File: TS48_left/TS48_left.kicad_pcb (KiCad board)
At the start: 2 copper layers, 124 x 77.9 mm, 123 parts, among them Q1 Q_NPN_BCE, SW1 SW_PUSH, U1 ATmega32U4, U2 PRTR5V0U2X, Y1 

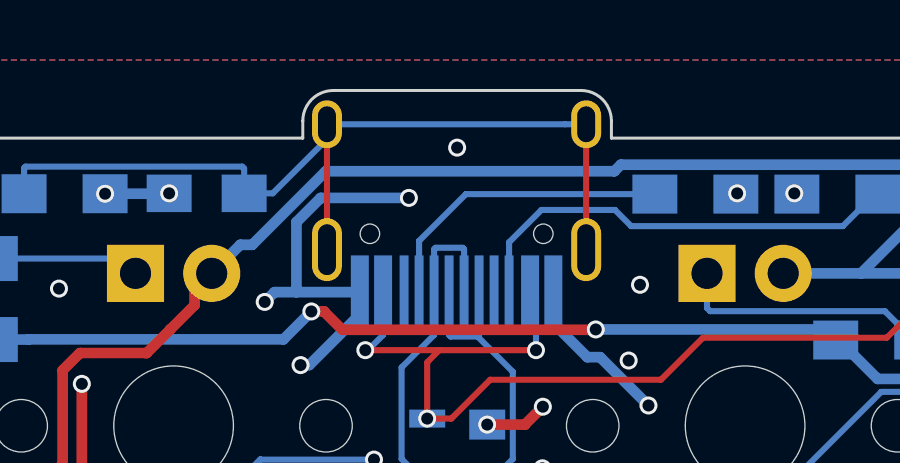
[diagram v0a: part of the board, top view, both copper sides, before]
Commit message: Gerbers
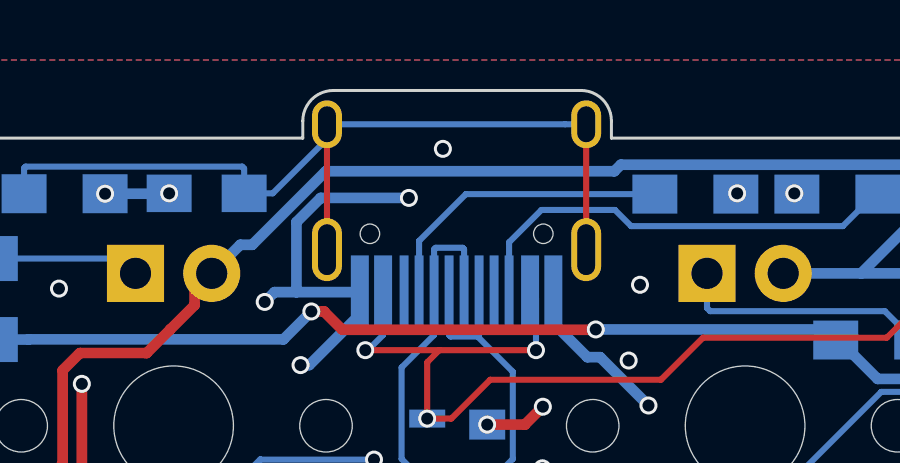
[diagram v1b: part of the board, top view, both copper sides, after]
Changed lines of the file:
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@@
-(kicad_pcb (version 20171130) (host pcbnew "(5.0.0)")
+(kicad_pcb (version 20171130) (host pcbnew "(6.0.0-rc1-dev-1291-g61b749f0b)")
   (general
     (thickness 1.6)
@@
     (zone_45_only no)
     (trace_min 0)
-    (segment_width 0.2)
-    (edge_width 0.1)
     (via_size 0.6)
     (via_drill 0.4)
@@
     (uvia_min_size 0.2)
     (uvia_min_drill 0.1)
+    (edge_width 0.1)
+    (segment_width 0.2)
     (pcb_text_width 0.3)
     (pcb_text_size 1.5 1.5)
@@
     (pad_drill 1.04)
     (pad_to_mask_clearance 0)
+    (solder_mask_min_width 0.25)
     (aux_axis_origin 0 0)
     (visible_elements 7FFFF7FF)
@@
       (layerselection 0x010fc_ffffffff)
       (usegerberextensions false)
-      (usegerberattributes false)
+      (usegerberattributes true)
       (usegerberadvancedattributes false)
       (creategerberjobfile false)
-      (excludeedgelayer true)
+      (excludeedgelayer false)
       (linewidth 0.100000)
       (plotframeref false)
@@
       (outputformat 1)
       (mirror false)
-      (drillshape 1)
+      (drillshape 0)
       (scaleselection 1)
       (outputdirectory ""))
@@
   (via (at 124.714 81.534) (size 0.6) (drill 0.4) (layers F.Cu B.Cu) (net 2))
   (via (at 111.887 80.772) (size 0.6) (drill 0.4) (layers F.Cu B.Cu) (net 2))
-  (via (at 109.0295 66.929) (size 0.6) (drill 0.4) (layers F.Cu B.Cu) (net 2))
+  (via (at 108.55452 66.96964) (size 0.6) (drill 0.4) (layers F.Cu B.Cu) (net 2))
   (via (at 115.1255 71.501) (size 0.6) (drill 0.4) (layers F.Cu B.Cu) (net 2))
   (via (at 102.616 72.0725) (size 0.6) (drill 0.4) (layers F.Cu B.Cu) (net 2))
